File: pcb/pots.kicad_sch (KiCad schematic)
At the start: 9 parts

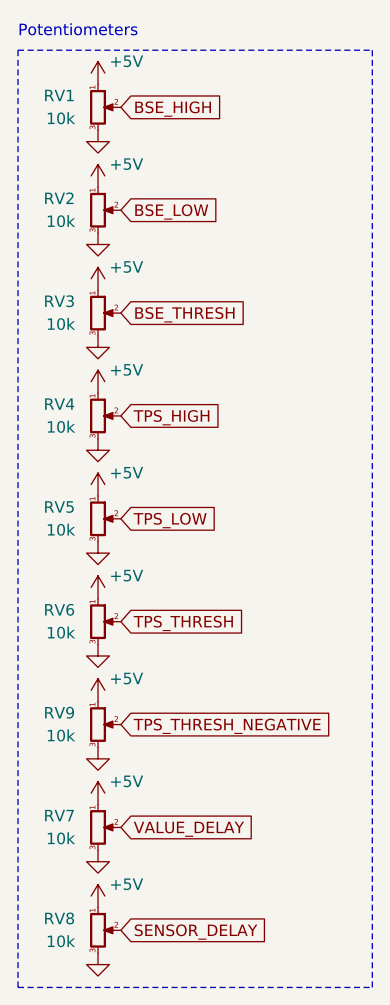
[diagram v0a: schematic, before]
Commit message: REV 8 Init
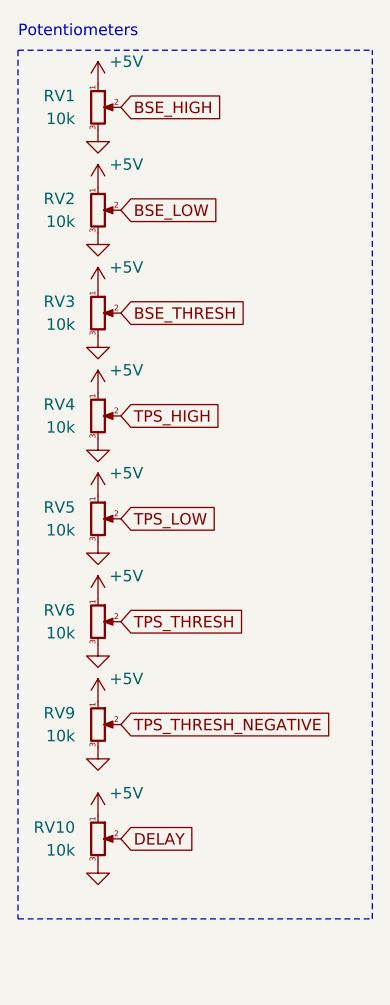
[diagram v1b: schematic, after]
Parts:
- removed RV7, RV8: 10k, Potentiometer_SMD:Potentiometer_Bourns_TC33X_Vertical, symbol Device:R_Potentiometer_Small
- added RV10: 10k, Potentiometer_SMD:Potentiometer_Bourns_TC33X_Vertical, symbol Device:R_Potentiometer_Small
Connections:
- net +5V: now also RV10.1
- net GND: now also RV10.3
- new net DELAY: RV10.2
